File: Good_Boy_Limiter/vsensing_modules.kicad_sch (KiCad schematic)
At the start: 20 parts, among them U10 B3B-XH-A, U11 B3B-XH-A, U12 B3B-XH-A, U8 B3B-XH-A

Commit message: Finished e-scheme
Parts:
- R1, R12, R16, R18: LCSC Part C177329 -> C25803
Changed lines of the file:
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@@
+			)
+		)
+		(property "Sim.Type" ""
+			(at 243.84 48.26 0)
+			(effects
+				(font
+					(size 1.27 1.27)
+				)
 			)
 		)
@@
 		)
 		(property "Sim.Device" ""
+			(at 114.3 80.01 0)
+			(effects
+				(font
+					(size 1.27 1.27)
+				)
+			)
+		)
+		(property "Sim.Type" ""
 			(at 114.3 80.01 0)
 			(effects
@@
 			)
 		)
+		(property "Sim.Type" ""
+			(at 233.68 80.01 0)
+			(effects
+				(font
+					(size 1.27 1.27)
+				)
+			)
+		)
 		(pin "2"
 		)
@@
 			)
 		)
+		(property "Sim.Type" ""
+			(at 250.19 92.71 0)
+			(effects
+				(font
+					(size 1.27 1.27)
+				)
+			)
+		)
 		(pin "2"
 		)
@@
 			)
 		)
+		(property "Sim.Type" ""
+			(at 193.04 92.71 0)
+			(effects
+				(font
+					(size 1.27 1.27)
+				)
+			)
+		)
 		(pin "2"
 		)
@@
 			)
 		)
+		(property "Sim.Type" ""
+			(at 242.57 59.69 0)
+			(effects
+				(font
+					(size 1.27 1.27)
+				)
+			)
+		)
 		(pin "3"
 		)
@@
 			)
 		)
+		(property "Sim.Type" ""
+			(at 185.42 59.69 0)
+			(effects
+				(font
+					(size 1.27 1.27)
+				)
+			)
+		)
 		(pin "3"
 		)
@@
 			)
 		)
+		(property "Sim.Type" ""
+			(at 66.04 92.71 0)
+			(effects
+				(font
+					(size 1.27 1.27)
+				)
+			)
+		)
 		(pin "2"
 		)
@@
 		)
 		(property "Sim.Device" ""
+			(at 49.53 80.01 0)
+			(effects
+				(font
+					(size 1.27 1.27)
+				)
+			)
+		)
+		(property "Sim.Type" ""
 			(at 49.53 80.01 0)
 			(effects
@@
 			)
 		)
-		(property "LCSC Part" "C177329"
+		(property "LCSC Part" "C25803"
 			(at 242.57 72.39 0)
 			(effects
@@
 		)
 		(property "Sim.Device" ""
+			(at 242.57 72.39 0)
+			(effects
+				(font
+					(size 1.27 1.27)
+				)
+			)
+		)
+		(property "Sim.Type" ""
 			(at 242.57 72.39 0)
 			(effects
@@
 			)
 		)
+		(property "Sim.Type" ""
+			(at 123.19 59.69 0)
+			(effects
+				(font
+					(size 1.27 1.27)
+				)
+			)
+		)
 		(pin "3"
 		)
@@
 			)
 		)
-		(property "LCSC Part" "C177329"
+		(property "LCSC Part" "C25803"
 			(at 58.42 72.39 0)
 			(effects
@@
 		)
 		(property "Sim.Device" ""
+			(at 58.42 72.39 0)
+			(effects
+				(font
+					(size 1.27 1.27)
+				)
+			)
+		)
+		(property "Sim.Type" ""
 			(at 58.42 72.39 0)
 			(effects
@@
 			)
 		)
+		(property "Sim.Type" ""
+			(at 186.69 48.26 0)
+			(effects
+				(font
+					(size 1.27 1.27)
+				)
+			)
+		)
 		(pin "2"
 		)
@@
 			)
 		)
-		(property "LCSC Part" "C177329"
+		(property "LCSC Part" "C25803"
 			(at 185.42 72.39 0)
 			(effects
@@
 		)
 		(property "Sim.Device" ""
+			(at 185.42 72.39 0)
+			(effects
+				(font
+					(size 1.27 1.27)
+				)
+			)
+		)
+		(property "Sim.Type" ""
 			(at 185.42 72.39 0)
 			(effects
@@
 			)
 		)
+		(property "Sim.Type" ""
+			(at 59.69 48.26 0)
+			(effects
+				(font
+					(size 1.27 1.27)
+				)
+			)
+		)
 		(pin "2"
 		)
@@
 			)
 		)
+		(property "Sim.Type" ""
+			(at 130.81 92.71 0)
+			(effects
+				(font
+					(size 1.27 1.27)
+				)
+			)
+		)
 		(pin "2"
 		)
@@
 			)
 		)
+		(property "Sim.Type" ""
+			(at 58.42 59.69 0)
+			(effects
+				(font
+					(size 1.27 1.27)
+				)
+			)
+		)
 		(pin "3"
 		)
@@
 		)
 		(property "Sim.Device" ""
+			(at 176.53 80.01 0)
+			(effects
+				(font
+					(size 1.27 1.27)
+				)
+			)
+		)
+		(property "Sim.Type" ""
 			(at 176.53 80.01 0)
 			(effects
@@
 			)
 		)
-		(property "LCSC Part" "C177329"
+		(property "LCSC Part" "C25803"
 			(at 123.19 72.39 0)
 			(effects
@@
 			)
 		)
+		(property "Sim.Type" ""
+			(at 123.19 72.39 0)
+			(effects
+				(font
+					(size 1.27 1.27)
+				)
+			)
+		)
 		(pin "2"
 		)
@@
 			(at 124.46 48.26 0)
 			(effects
+				(font
+					(size 1.27 1.27)
+				)
+			)
+		)
+		(property "Sim.Type" ""
+			(at 124.46 48.26 0)
+			(effects

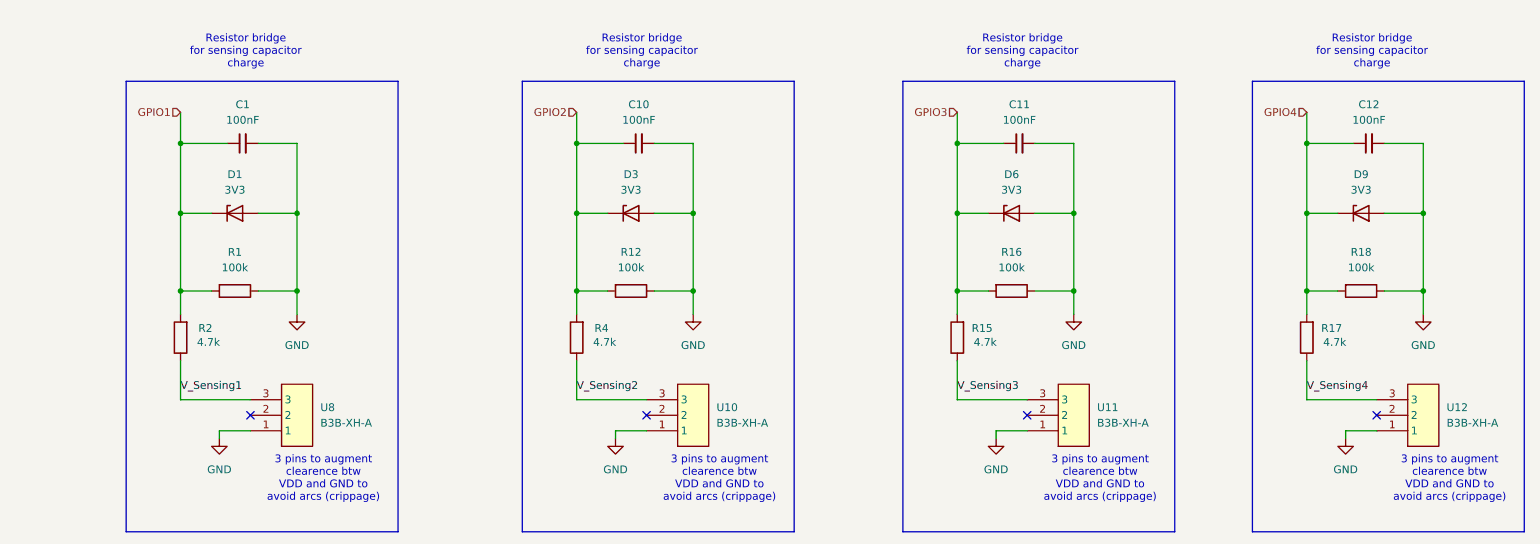
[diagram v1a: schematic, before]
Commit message: started routing
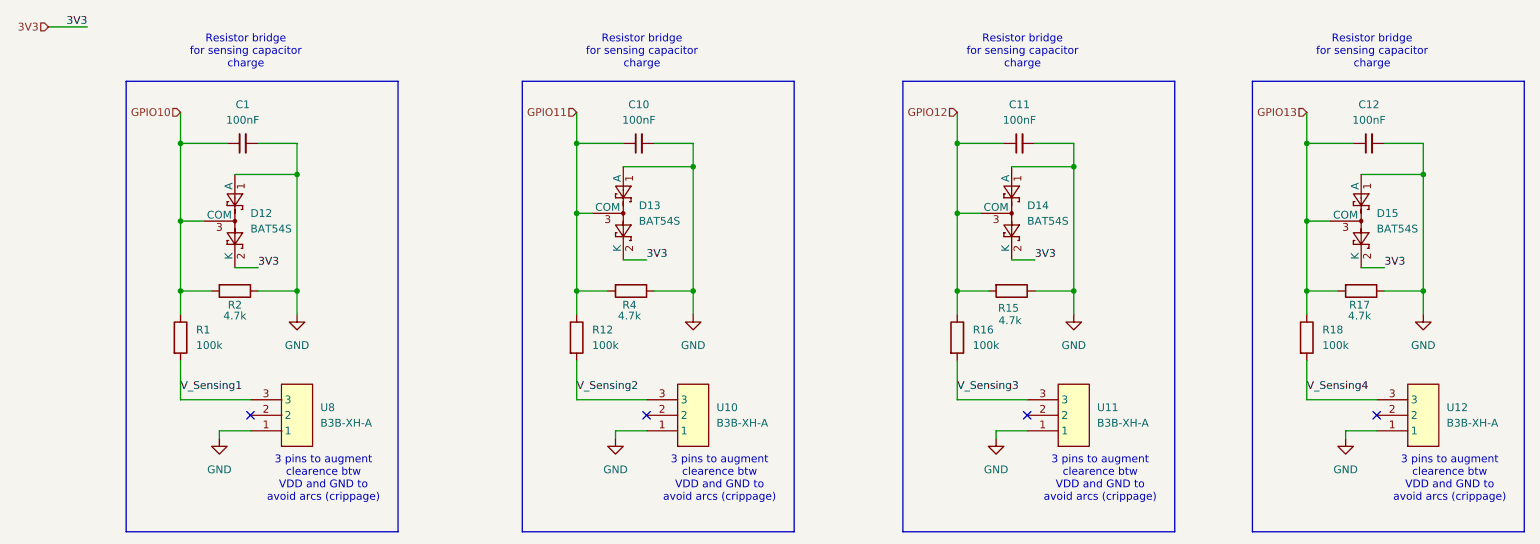
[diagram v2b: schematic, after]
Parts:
- removed D1, D3, D6, D9: 3V3, Package_TO_SOT_SMD:SOT-23, symbol Diode:BZX84Cxx
- added D12, D13, D14, D15: BAT54S, Package_TO_SOT_SMD:SOT-23, symbol Diode:BAT54S
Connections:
- net GND: now also R15.1, R17.1, R2.1, R4.1, D12.1 (A), D13.1 (A), D14.1 (A), D15.1 (A); no longer R1.1, R12.1, R16.1, R18.1
- net V_Sensing1: now also R1.2; no longer R2.1
- net V_Sensing2: now also R12.2; no longer R4.1
- net V_Sensing3: now also R16.2; no longer R15.1
- net V_Sensing4: now also R18.2; no longer R17.1
- net GPIO1 renamed GPIO10
- net GPIO10: now also R1.1, D12.3 (COM); no longer R1.2
- net GPIO2 renamed GPIO11
- net GPIO11: now also R12.1, D13.3 (COM); no longer R12.2
- net GPIO3 renamed GPIO12
- net GPIO12: now also R16.1, D14.3 (COM); no longer R16.2
- net GPIO4 renamed GPIO13
- net GPIO13: now also R18.1, D15.3 (COM); no longer R18.2
- new net 3V3: D12.2 (K), D13.2 (K), D14.2 (K), D15.2 (K)
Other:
- moved on the sheet: R1, R12, R15, R16, R17, R18, R2, R4
